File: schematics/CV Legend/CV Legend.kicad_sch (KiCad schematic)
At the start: 1 part

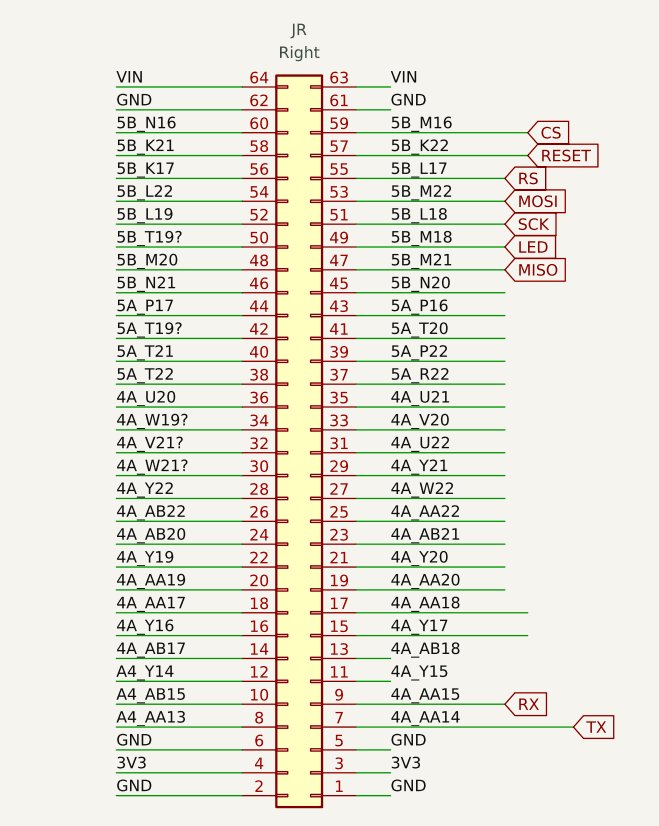
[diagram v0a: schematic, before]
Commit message: Rv32: Some schematics work.
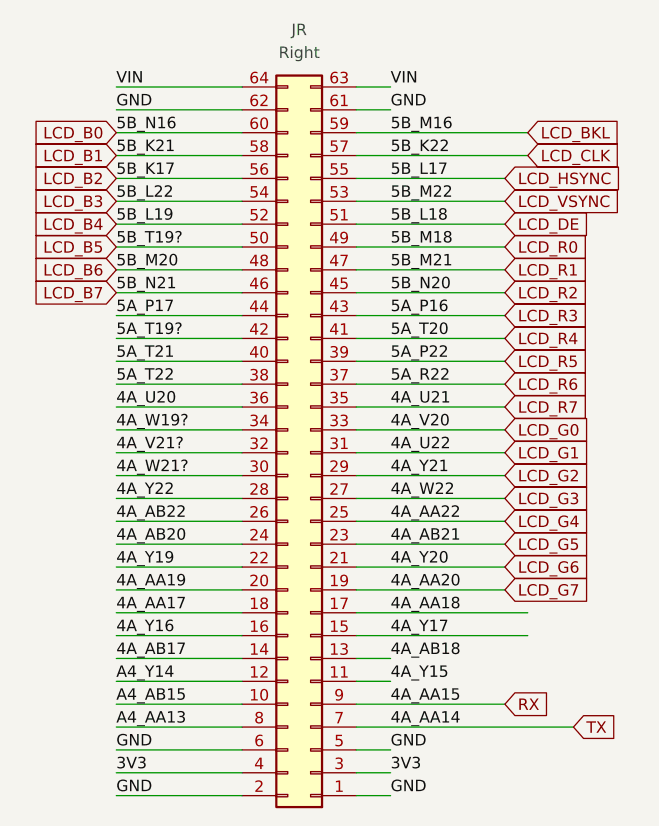
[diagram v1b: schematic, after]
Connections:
- net 4A_AA20 renamed LCD_G7
- net 4A_AA22 renamed LCD_G4
- net 4A_AB21 renamed LCD_G5
- net 4A_U21 renamed LCD_R7
- net 4A_U22 renamed LCD_G1
- net 4A_V20 renamed LCD_G0
- net 4A_W22 renamed LCD_G3
- net 4A_Y20 renamed LCD_G6
- net 4A_Y21 renamed LCD_G2
- net 5A_P16 renamed LCD_R3
- net 5A_P22 renamed LCD_R5
- net 5A_R22 renamed LCD_R6
- net 5A_T20 renamed LCD_R4
- net 5B_K17 renamed LCD_B2
- net 5B_K21 renamed LCD_B1
- net 5B_L19 renamed LCD_B4
- net 5B_L22 renamed LCD_B3
- net 5B_M20 renamed LCD_B6
- net 5B_N16 renamed LCD_B0
- net 5B_N20 renamed LCD_R2
- net 5B_N21 renamed LCD_B7
- net 5B_T19? renamed LCD_B5
- net CS renamed LCD_BKL
- net LED renamed LCD_R0
- net MISO renamed LCD_R1
- net MOSI renamed LCD_VSYNC
- net RESET renamed LCD_CLK
- net RS renamed LCD_HSYNC
- net SCK renamed LCD_DE
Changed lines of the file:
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@@
     (effects (font (size 1.27 1.27)) (justify left bottom))
   )
-  (global_label "MISO" (shape input) (at 140.97 64.77 0) (fields_autoplaced)
+  (global_label "LCD_B3" (shape input) (at 97.79 57.15 180) (fields_autoplaced)
+    (effects (font (size 1.27 1.27)) (justify right))
+    (property "Intersheet References" "${INTERSHEET_REFS}" (id 0) (at 88.3617 57.0706 0)
+      (effects (font (size 1.27 1.27)) (justify right) hide)
+    )
+  )
+  (global_label "LCD_R3" (shape input) (at 140.97 69.85 0) (fields_autoplaced)
     (effects (font (size 1.27 1.27)) (justify left))
-    (property "Intersheet References" "${INTERSHEET_REFS}" (id 0) (at 147.9793 64.6906 0)
+    (property "Intersheet References" "${INTERSHEET_REFS}" (id 0) (at 150.3983 69.7706 0)
       (effects (font (size 1.27 1.27)) (justify left) hide)
     )
   )
-  (global_label "CS" (shape input) (at 143.51 49.53 0) (fields_autoplaced)
+  (global_label "LCD_G4" (shape input) (at 140.97 92.71 0) (fields_autoplaced)
     (effects (font (size 1.27 1.27)) (justify left))
-    (property "Intersheet References" "${INTERSHEET_REFS}" (id 0) (at 148.4026 49.4506 0)
+    (property "Intersheet References" "${INTERSHEET_REFS}" (id 0) (at 150.3983 92.6306 0)
+      (effects (font (size 1.27 1.27)) (justify left) hide)
+    )
+  )
+  (global_label "LCD_R6" (shape input) (at 140.97 77.47 0) (fields_autoplaced)
+    (effects (font (size 1.27 1.27)) (justify left))
+    (property "Intersheet References" "${INTERSHEET_REFS}" (id 0) (at 150.3983 77.3906 0)
+      (effects (font (size 1.27 1.27)) (justify left) hide)
+    )
+  )
+  (global_label "LCD_G0" (shape input) (at 140.97 82.55 0) (fields_autoplaced)
+    (effects (font (size 1.27 1.27)) (justify left))
+    (property "Intersheet References" "${INTERSHEET_REFS}" (id 0) (at 150.3983 82.4706 0)
+      (effects (font (size 1.27 1.27)) (justify left) hide)
+    )
+  )
+  (global_label "LCD_BKL" (shape input) (at 143.51 49.53 0) (fields_autoplaced)
+    (effects (font (size 1.27 1.27)) (justify left))
+    (property "Intersheet References" "${INTERSHEET_REFS}" (id 0) (at 154.0269 49.4506 0)
       (effects (font (size 1.27 1.27)) (justify left) hide)
     )
@@
     )
   )
-  (global_label "RS" (shape input) (at 140.97 54.61 0) (fields_autoplaced)
+  (global_label "LCD_R0" (shape input) (at 140.97 62.23 0) (fields_autoplaced)
     (effects (font (size 1.27 1.27)) (justify left))
-    (property "Intersheet References" "${INTERSHEET_REFS}" (id 0) (at 145.8626 54.5306 0)
+    (property "Intersheet References" "${INTERSHEET_REFS}" (id 0) (at 150.3983 62.1506 0)
       (effects (font (size 1.27 1.27)) (justify left) hide)
     )
   )
-  (global_label "SCK" (shape input) (at 140.97 59.69 0) (fields_autoplaced)
+  (global_label "LCD_HSYNC" (shape input) (at 140.97 54.61 0) (fields_autoplaced)
     (effects (font (size 1.27 1.27)) (justify left))
-    (property "Intersheet References" "${INTERSHEET_REFS}" (id 0) (at 147.1326 59.6106 0)
+    (property "Intersheet References" "${INTERSHEET_REFS}" (id 0) (at 154.1479 54.5306 0)
       (effects (font (size 1.27 1.27)) (justify left) hide)
     )
   )
-  (global_label "RESET" (shape input) (at 143.51 52.07 0) (fields_autoplaced)
+  (global_label "LCD_G3" (shape input) (at 140.97 90.17 0) (fields_autoplaced)
     (effects (font (size 1.27 1.27)) (justify left))
-    (property "Intersheet References" "${INTERSHEET_REFS}" (id 0) (at 151.6683 51.9906 0)
+    (property "Intersheet References" "${INTERSHEET_REFS}" (id 0) (at 150.3983 90.0906 0)
       (effects (font (size 1.27 1.27)) (justify left) hide)
     )
   )
-  (global_label "MOSI" (shape input) (at 140.97 57.15 0) (fields_autoplaced)
+  (global_label "LCD_B1" (shape input) (at 97.79 52.07 180) (fields_autoplaced)
+    (effects (font (size 1.27 1.27)) (justify right))
+    (property "Intersheet References" "${INTERSHEET_REFS}" (id 0) (at 88.3617 51.9906 0)
+      (effects (font (size 1.27 1.27)) (justify right) hide)
+    )
+  )
+  (global_label "LCD_R7" (shape input) (at 140.97 80.01 0) (fields_autoplaced)
     (effects (font (size 1.27 1.27)) (justify left))
-    (property "Intersheet References" "${INTERSHEET_REFS}" (id 0) (at 147.9793 57.0706 0)
+    (property "Intersheet References" "${INTERSHEET_REFS}" (id 0) (at 150.3983 79.9306 0)
       (effects (font (size 1.27 1.27)) (justify left) hide)
+    )
+  )
+  (global_label "LCD_DE" (shape input) (at 140.97 59.69 0) (fields_autoplaced)
+    (effects (font (size 1.27 1.27)) (justify left))
+    (property "Intersheet References" "${INTERSHEET_REFS}" (id 0) (at 150.3379 59.6106 0)
+      (effects (font (size 1.27 1.27)) (justify left) hide)
+    )
+  )
+  (global_label "LCD_G2" (shape input) (at 140.97 87.63 0) (fields_autoplaced)
+    (effects (font (size 1.27 1.27)) (justify left))
+    (property "Intersheet References" "${INTERSHEET_REFS}" (id 0) (at 150.3983 87.5506 0)
+      (effects (font (size 1.27 1.27)) (justify left) hide)
+    )
+  )
+  (global_label "LCD_R5" (shape input) (at 140.97 74.93 0) (fields_autoplaced)
+    (effects (font (size 1.27 1.27)) (justify left))
+    (property "Intersheet References" "${INTERSHEET_REFS}" (id 0) (at 150.3983 74.8506 0)
+      (effects (font (size 1.27 1.27)) (justify left) hide)
+    )
+  )
+  (global_label "LCD_B5" (shape input) (at 97.79 62.23 180) (fields_autoplaced)
+    (effects (font (size 1.27 1.27)) (justify right))
+    (property "Intersheet References" "${INTERSHEET_REFS}" (id 0) (at 88.3617 62.1506 0)
+      (effects (font (size 1.27 1.27)) (justify right) hide)
+    )
+  )
+  (global_label "LCD_CLK" (shape input) (at 143.51 52.07 0) (fields_autoplaced)
+    (effects (font (size 1.27 1.27)) (justify left))
+    (property "Intersheet References" "${INTERSHEET_REFS}" (id 0) (at 154.0269 51.9906 0)
+      (effects (font (size 1.27 1.27)) (justify left) hide)
+    )
+  )
+  (global_label "LCD_G6" (shape input) (at 140.97 97.79 0) (fields_autoplaced)
+    (effects (font (size 1.27 1.27)) (justify left))
+    (property "Intersheet References" "${INTERSHEET_REFS}" (id 0) (at 150.3983 97.7106 0)
+      (effects (font (size 1.27 1.27)) (justify left) hide)
+    )
+  )
+  (global_label "LCD_VSYNC" (shape input) (at 140.97 57.15 0) (fields_autoplaced)
+    (effects (font (size 1.27 1.27)) (justify left))
+    (property "Intersheet References" "${INTERSHEET_REFS}" (id 0) (at 153.906 57.0706 0)
+      (effects (font (size 1.27 1.27)) (justify left) hide)
+    )
+  )
+  (global_label "LCD_B0" (shape input) (at 97.79 49.53 180) (fields_autoplaced)
+    (effects (font (size 1.27 1.27)) (justify right))
+    (property "Intersheet References" "${INTERSHEET_REFS}" (id 0) (at 88.3617 49.4506 0)
+      (effects (font (size 1.27 1.27)) (justify right) hide)
+    )
+  )
+  (global_label "LCD_B7" (shape input) (at 97.79 67.31 180) (fields_autoplaced)
+    (effects (font (size 1.27 1.27)) (justify right))
+    (property "Intersheet References" "${INTERSHEET_REFS}" (id 0) (at 88.3617 67.2306 0)
+      (effects (font (size 1.27 1.27)) (justify right) hide)
+    )
+  )
+  (global_label "LCD_R2" (shape input) (at 140.97 67.31 0) (fields_autoplaced)
+    (effects (font (size 1.27 1.27)) (justify left))
+    (property "Intersheet References" "${INTERSHEET_REFS}" (id 0) (at 150.3983 67.2306 0)
+      (effects (font (size 1.27 1.27)) (justify left) hide)
+    )
+  )
+  (global_label "LCD_B4" (shape input) (at 97.79 59.69 180) (fields_autoplaced)
+    (effects (font (size 1.27 1.27)) (justify right))
+    (property "Intersheet References" "${INTERSHEET_REFS}" (id 0) (at 88.3617 59.6106 0)
+      (effects (font (size 1.27 1.27)) (justify right) hide)
     )
   )
@@
     )
   )
-  (global_label "LED" (shape input) (at 140.97 62.23 0) (fields_autoplaced)
+  (global_label "LCD_G5" (shape input) (at 140.97 95.25 0) (fields_autoplaced)
     (effects (font (size 1.27 1.27)) (justify left))
-    (property "Intersheet References" "${INTERSHEET_REFS}" (id 0) (at 146.8302 62.1506 0)
+    (property "Intersheet References" "${INTERSHEET_REFS}" (id 0) (at 150.3983 95.1706 0)
       (effects (font (size 1.27 1.27)) (justify left) hide)
     )
+  )
+  (global_label "LCD_G1" (shape input) (at 140.97 85.09 0) (fields_autoplaced)
+    (effects (font (size 1.27 1.27)) (justify left))
+    (property "Intersheet References" "${INTERSHEET_REFS}" (id 0) (at 150.3983 85.0106 0)
+      (effects (font (size 1.27 1.27)) (justify left) hide)
+    )
+  )
+  (global_label "LCD_B2" (shape input) (at 97.79 54.61 180) (fields_autoplaced)
+    (effects (font (size 1.27 1.27)) (justify right))
+    (property "Intersheet References" "${INTERSHEET_REFS}" (id 0) (at 88.3617 54.5306 0)
+      (effects (font (size 1.27 1.27)) (justify right) hide)
+    )
+  )
+  (global_label "LCD_B6" (shape input) (at 97.79 64.77 180) (fields_autoplaced)
+    (effects (font (size 1.27 1.27)) (justify right))
+    (property "Intersheet References" "${INTERSHEET_REFS}" (id 0) (at 88.3617 64.6906 0)
+      (effects (font (size 1.27 1.27)) (justify right) hide)
+    )
+  )
+  (global_label "LCD_G7" (shape input) (at 140.97 100.33 0) (fields_autoplaced)
+    (effects (font (size 1.27 1.27)) (justify left))
+    (property "Intersheet References" "${INTERSHEET_REFS}" (id 0) (at 150.3983 100.2506 0)
+      (effects (font (size 1.27 1.27)) (justify left) hide)
+    )
+  )
+  (global_label "LCD_R4" (shape input) (at 140.97 72.39 0) (fields_autoplaced)
+    (effects (font (size 1.27 1.27)) (justify left))
+    (property "Intersheet References" "${INTERSHEET_REFS}" (id 0) (at 150.3983 72.3106 0)
+      (effects (font (size 1.27 1.27)) (justify left) hide)
+    )
+  )
+  (global_label "LCD_R1" (shape input) (at 140.97 64.77 0) (fields_autoplaced)
+    (effects (font (size 1.27 1.27)) (justify left))
+    (property "Intersheet References" "${INTERSHEET_REFS}" (id 0) (at 150.3983 64.6906 0)
+      (effects (font (size 1.27 1.27)) (justify left) hide)
+    )
